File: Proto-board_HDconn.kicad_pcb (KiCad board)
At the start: 2 copper layers, 88.9 x 127 mm, 102 parts, among them J1 Conn_01x02, J2 Conn_01x06, J3 Conn_01x05, J4 Conn_01x05, J5 Conn_01x05, J6 Conn_01x05, J7 Conn_01x16, J9 Conn_02x06_Odd_Even, SW1 9001-XX-00, SW10 9001-XX-00, SW11 9001-XX-00, SW12 9001-XX-00, SW13 9001-XX-00, SW14 9001-XX-00, SW15 9001-XX-00, SW16 9001-XX-00, SW17 9001-XX-00, SW18 9001-XX-00, SW19 9001-XX-00, SW2 9001-XX-00, SW20 9001-XX-00, SW3 9001-XX-00, SW4 9001-XX-00, SW5 9001-XX-00, SW6 9001-XX-00, SW7 9001-XX-00, SW8 9001-XX-00, SW9 9001-XX-00, U1 TPL7407LA, U2 MAX17502, U3 XC2C128-VQ100, U4 TPL7407LA, U5 TPL7407LA, U6 MAX15027

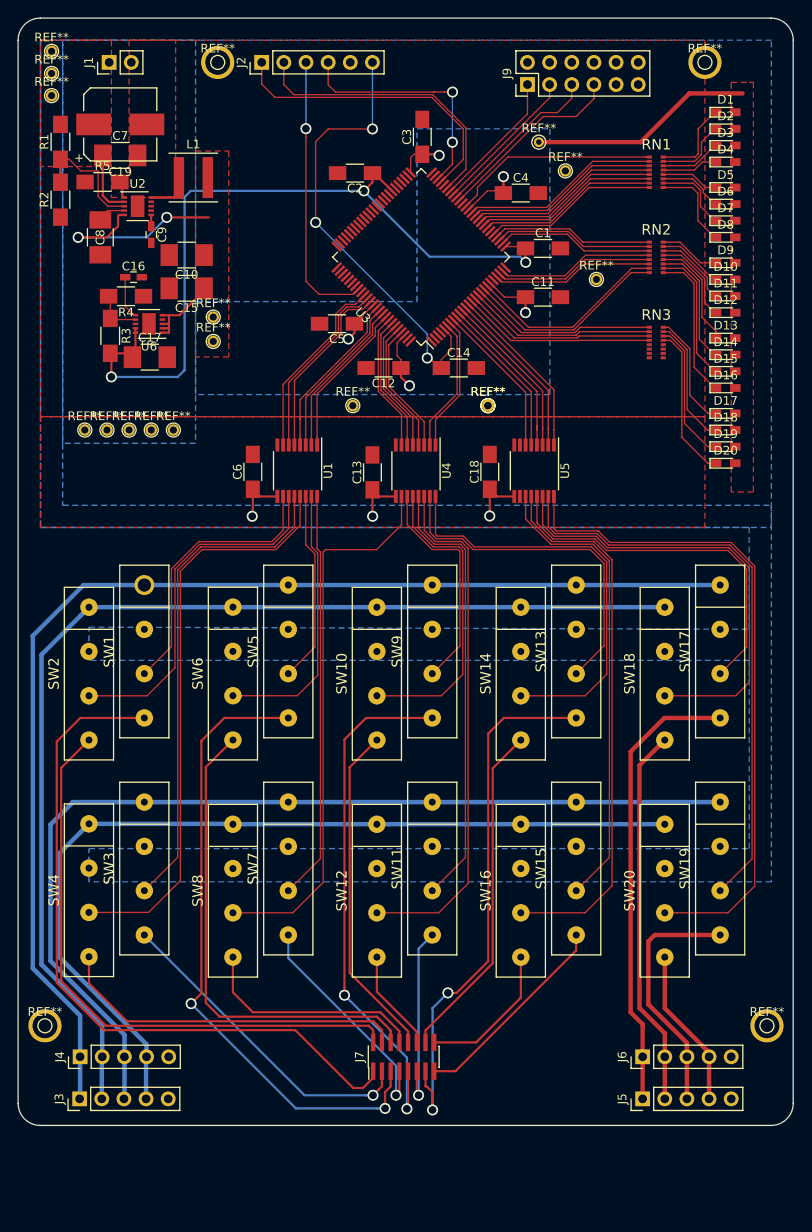
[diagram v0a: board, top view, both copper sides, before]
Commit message: Final version of protoboard prior to major revision.
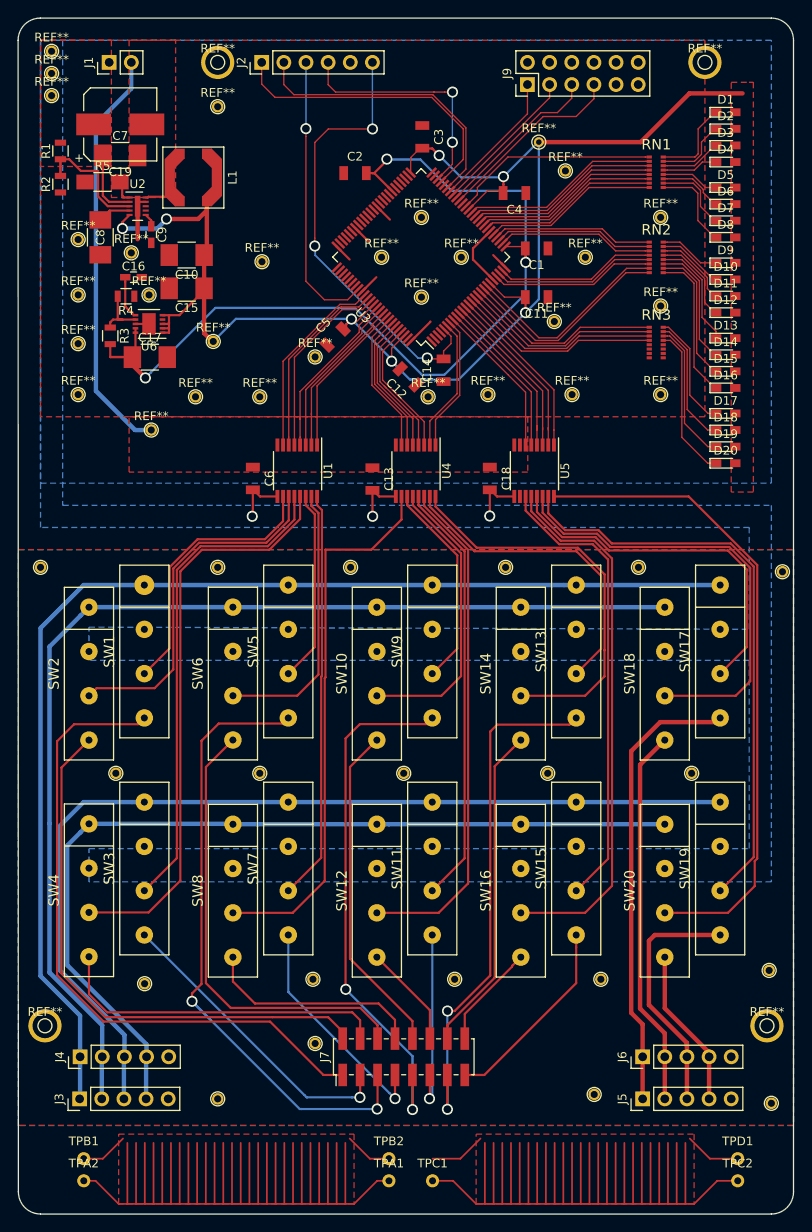
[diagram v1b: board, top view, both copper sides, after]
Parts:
- removed the REF** at (177.1, 130.6)
- removed the REF** at (174.5, 130.6)
- removed the REF** at (172.0, 130.6)
- removed the REF** at (186.7, 117.6)
- removed the REF** at (218.2, 127.8)
- removed the REF** at (182.2, 130.6)
- added REF**: PINTST, Connectors:PINTST, F.Cu at (184.7, 126.7)
- added REF**: PINTST, Connectors:PINTST, F.Cu at (250.5, 192.5)
- added REF**: PINTST, Connectors:PINTST, F.Cu at (252.0, 146.8)
- added REF**: PINTST, Connectors:PINTST, F.Cu at (230.4, 206.8)
- added REF**: PINTST, Connectors:PINTST, F.Cu at (187.2, 207.3)
- added REF**: PINTST, Connectors:PINTST, F.Cu at (198.4, 200.9)
- added REF**: PINTST, Connectors:PINTST, F.Cu at (231.2, 193.5)
- added REF**: PINTST, Connectors:PINTST, F.Cu at (214.4, 193.5)
- added REF**: PINTST, Connectors:PINTST, F.Cu at (198.2, 193.5)
- added REF**: PINTST, Connectors:PINTST, F.Cu at (178.8, 194.1)
- added REF**: PINTST, Connectors:PINTST, F.Cu at (241.6, 169.9)
- added REF**: PINTST, Connectors:PINTST, F.Cu at (192.1, 126.7)
- added REF**: PINTST, Connectors:PINTST, F.Cu at (225.1, 169.9)
- added REF**: PINTST, Connectors:PINTST, F.Cu at (175.5, 169.9)
- added REF**: PINTST, Connectors:PINTST, F.Cu at (192.1, 169.9)
- added REF**: PINTST, Connectors:PINTST, F.Cu at (208.6, 169.9)
- added REF**: PINTST, Connectors:PINTST, F.Cu at (235.5, 146.3)
- added REF**: PINTST, Connectors:PINTST, F.Cu at (220.2, 146.3)
- added REF**: PINTST, Connectors:PINTST, F.Cu at (202.5, 146.3)
- added REF**: PINTST, Connectors:PINTST, F.Cu at (187.2, 146.3)
- added REF**: PINTST, Connectors:PINTST, F.Cu at (166.9, 146.3)
- added REF**: PINTST, Connectors:PINTST, F.Cu at (198.4, 122.2)
- added REF**: PINTST, Connectors:PINTST, F.Cu at (171.2, 126.5)
- added REF**: PINTST, Connectors:PINTST, F.Cu at (187.2, 93.5)
- added REF**: PINTST, Connectors:PINTST, F.Cu at (192.3, 111.3)
- added REF**: PINTST, Connectors:PINTST, F.Cu at (238.0, 106.2)
- added REF**: PINTST, Connectors:PINTST, F.Cu at (238.0, 116.3)
- added REF**: PINTST, Connectors:PINTST, F.Cu at (238.0, 126.5)
- added REF**: PINTST, Connectors:PINTST, F.Cu at (227.9, 126.5)
- added REF**: PINTST, Connectors:PINTST, F.Cu at (229.4, 110.7)
- added REF**: PINTST, Connectors:PINTST, F.Cu at (210.6, 115.3)
- added REF**: PINTST, Connectors:PINTST, F.Cu at (215.2, 110.7)
- added REF**: PINTST, Connectors:PINTST, F.Cu at (171.2, 120.7)
- added REF**: PINTST, Connectors:PINTST, F.Cu at (206.0, 110.7)
- added REF**: PINTST, Connectors:PINTST, F.Cu at (210.6, 106.2)
- added REF**: PINTST, Connectors:PINTST, F.Cu at (179.4, 115.1)
- added REF**: PINTST, Connectors:PINTST, F.Cu at (171.2, 115.1)
- added REF**: PINTST, Connectors:PINTST, F.Cu at (171.2, 108.7)
- added REF**: PINTST, Connectors:PINTST, F.Cu at (177.3, 110.2)
- added REF**: PINTST, Connectors:PINTST, F.Cu at (250.7, 207.8)
- added TPA1: TEST, Measurement_Points:Measurement_Point_Round-TH_Small, F.Cu at (206.9, 216.7)
- added TPA2: TEST, Measurement_Points:Measurement_Point_Round-TH_Small, F.Cu at (171.9, 216.7)
- added TPB1: TEST, Measurement_Points:Measurement_Point_Round-TH_Small, F.Cu at (171.9, 214.1)
- added TPB2: TEST, Measurement_Points:Measurement_Point_Round-TH_Small, F.Cu at (206.9, 214.1)
- added TPC1: TEST, Measurement_Points:Measurement_Point_Round-TH_Small, F.Cu at (211.9, 216.7)
- added TPC2: TEST, Measurement_Points:Measurement_Point_Round-TH_Small, F.Cu at (246.9, 216.7)
- added TPD1: TEST, Measurement_Points:Measurement_Point_Round-TH_Small, F.Cu at (246.9, 214.1)
- C1, C11, C12, C13, C14, C18, C2, C3, C4, C5, C6: footprint Capacitors_SMD:C_1206_HandSoldering -> passives_IKM:1206_PROTO
- J7: footprint Pin_Headers:Pin_Header_Straight_2x08_Pitch1.00mm_SMD -> Pin_Headers:Pin_Header_Straight_2x08_Pitch2.00mm_SMD
- L1: footprint Inductors_SMD:L_Coilcraft_XAL5030 -> coilcraft_IKM:LPS6235
- R1, R2, R3, R4: footprint Resistors_SMD:R_1206_HandSoldering -> Resistors_SMD:R_0805
- U2: footprint Housings_DFN_QFN:DFN-10-1EP_3x3mm_Pitch0.5mm -> Housings_DFN_QFN:DFN-10-1EP_2x3mm_Pitch0.5mm
- moved REF** 8.70 mm to (211.4, 126.7)
- moved REF** 6.82 mm to (225.8, 118.1)
- moved C12 3.00 mm to (209.1, 124.5), turned to 315 degrees
- moved R2 1.78 mm to (169.2, 102.4)
- moved C14 1.76 mm to (213.1, 123.7), turned to 270 degrees
- moved C5 1.54 mm to (200.7, 119.9), turned to 225 degrees
- moved REF** 1.27 mm to (218.2, 126.5)
- moved R1 1.05 mm to (169.2, 98.6)
- moved C13 0.76 mm to (205.0, 136.2)
- moved C18 0.76 mm to (218.4, 136.1)
- moved C6 0.76 mm to (191.3, 136.1)
- moved C4 0.73 mm to (221.3, 103.4)
- moved C1 0.73 mm to (223.8, 109.7)
- moved C11 0.73 mm to (223.8, 115.3)
- turned L1 to 90 degrees
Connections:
- J3 pad 5: GNDREF -> GNDS
- J4 pad 5: GNDREF -> GNDS
- J5 pad 5: GNDREF -> GNDS
- J6 pad 5: GNDREF -> GNDS
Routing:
- net /TA+: track 0.00 -> 219.2 mm
- net /TB+: track 0.00 -> 205.2 mm
- net /3V3: track 89.3 -> 173.4 mm
- net GND: track 2.37 -> 50.7 mm
- net GNDREF: track 0.00 -> 29.1 mm
- net /1V8: track 89.9 -> 106.0 mm
- net /TA-: track 0.00 -> 10.9 mm
- net /TB-: track 0.00 -> 6.46 mm
- net (no net): track 0.00 -> 6.46 mm
- net /SS1.1: track 81.4 -> 75.4 mm
- net /SS4.4: track 16.7 -> 12.0 mm
- net /SS1.2: track 68.5 -> 63.9 mm
- net /SW4.1: track 39.5 -> 36.5 mm
- net /SW4.2: track 49.0 -> 46.0 mm
- net /SS2.2: track 55.3 -> 52.4 mm
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- added copper zone on F.Cu, net /TA-
- added copper zone on F.Cu, net /TB-
- added copper zone on B.Cu, net GNDS
- added copper zone on F.Cu, net GNDS
- removed copper zone on B.Cu, net /3V3
- removed copper zone on B.Cu, net GND
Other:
- board size 88.9 x 127 mm -> 88.9 x 137.2 mm
- rule trace_min: 0.1524 -> 0.152
- board text removed: "SMU"
